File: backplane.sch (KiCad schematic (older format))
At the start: 29 parts, among them J100 SEPERATION_SW, J105 +X SOLAR PANEL, J106 -X SOLAR PANEL, J107 +Y SOLAR PANEL, J200_1 HSEC8-160-01-S-DV-A-K-TR, J200_2 HSEC8-160-01-S-DV-A-K-TR, J200_3 HSEC8-160-01-S-DV-A-K-TR, J200_4 HSEC8-160-01-S-DV-A-K-TR, J200_5 HSEC8-160-01-S-DV-A-K-TR, J200_6 HSEC8-160-01-S-DV-A-K-TR, J200_7 HSEC8-160-01-S-DV-A-K-TR, J200_8 HSEC8-160-01-S-DV-A-K-TR, J300 Breakout Connector, J301 Breakout Connector, SW100 RESET, SW101 RESET

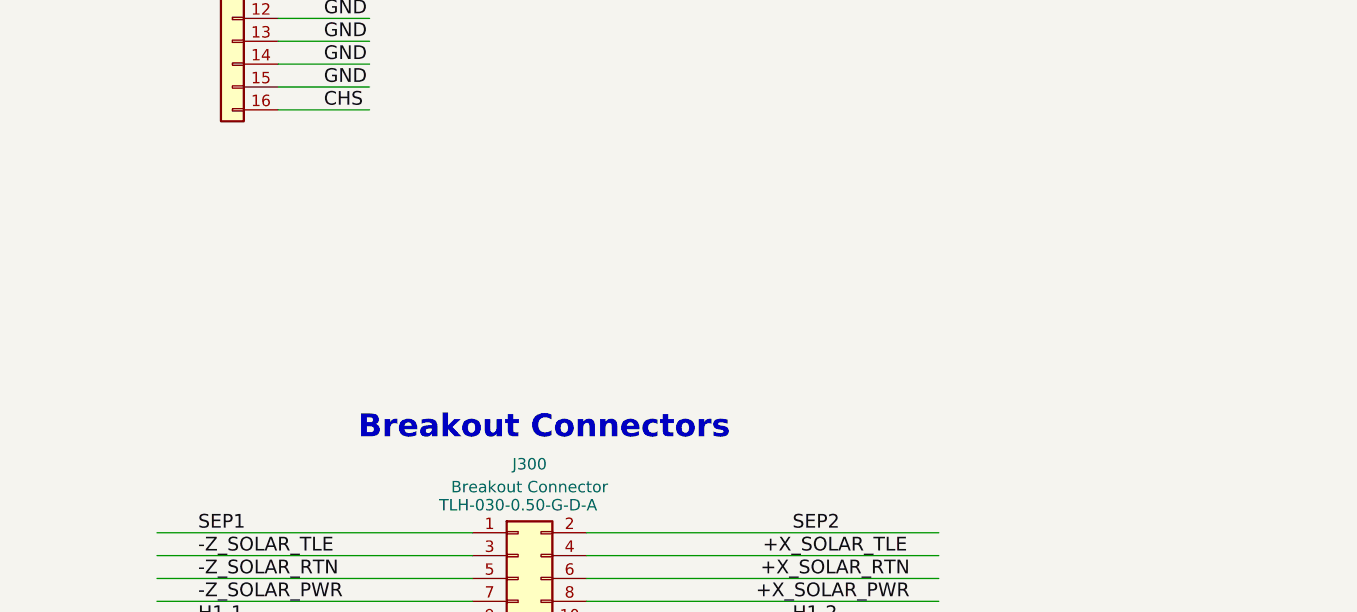
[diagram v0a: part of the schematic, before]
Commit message: final changes before ordering
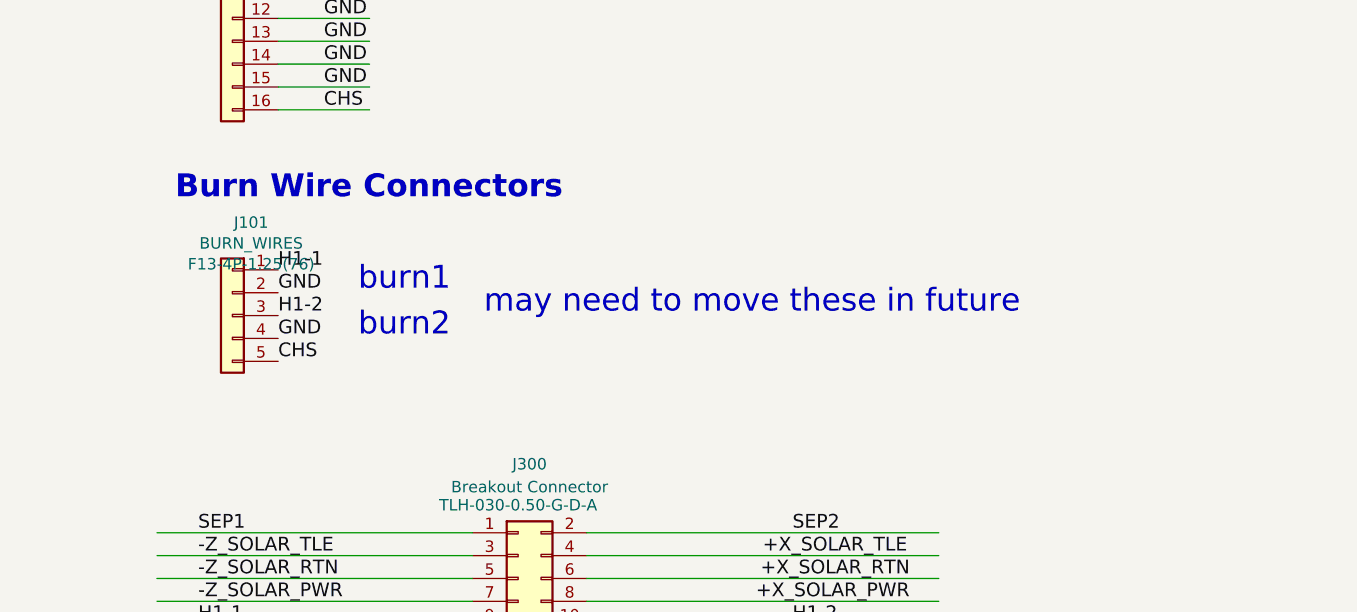
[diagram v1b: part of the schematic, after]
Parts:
- added J101: BURN_WIRES, CubeSat_Backplane:DF13-4P-1.25(75), symbol Connector_Generic:Conn_01x05
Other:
- note added: "Burn Wire Connectors"
- note added: "burn1"
- note added: "burn2"
- note added: "may need to move these in future"
- note removed: "Breakout Connectors"
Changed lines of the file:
@@
 Text Notes 13150 13900 0    100  ~ 0
 CHS, GND Jumper
-Text Notes 18150 4500 0    100  ~ 20
-Breakout Connectors
+Text Notes 17350 3450 0    100  ~ 20
+Burn Wire Connectors
 $Comp
 L Connector_Generic:Conn_02x30_Odd_Even J301
@@
 Text Notes 17400 15500 0    100  ~ 20
 BACKPLANE
+$Comp
+L Connector_Generic:Conn_01x05 J101
+U 1 1 61E229FD
+P 17600 3950
+F 0 "J101" H 17518 4357 50  0000 C CNN
+F 1 "BURN_WIRES" H 17518 4266 50  0000 C CNN
+F 2 "CubeSat_Backplane:DF13-4P-1.25(75)" H 17600 3950 50  0001 C CNN
+F 3 "F13-4P-1.25(76)" H 17518 4175 50  0000 C CNN
+	1    17600 3950
+	-1   0    0    -1
+$EndComp
+Text Label 17800 4050 0    60   ~ 0
+GND
+Text Label 17800 3850 0    60   ~ 0
+GND
+Text Label 17800 3750 0    60   ~ 0
+H1-1
+Text Label 17800 3950 0    60   ~ 0
+H1-2
+Text Notes 18150 3850 0    100  ~ 0
+burn1
+Text Notes 18150 4050 0    100  ~ 0
+burn2
+Text Notes 18700 3950 0    100  ~ 0
+may need to move these in future
+Text Label 17800 4150 0    60   ~ 0
+CHS
 $EndSCHEMATC
